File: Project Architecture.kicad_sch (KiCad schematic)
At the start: 0 parts

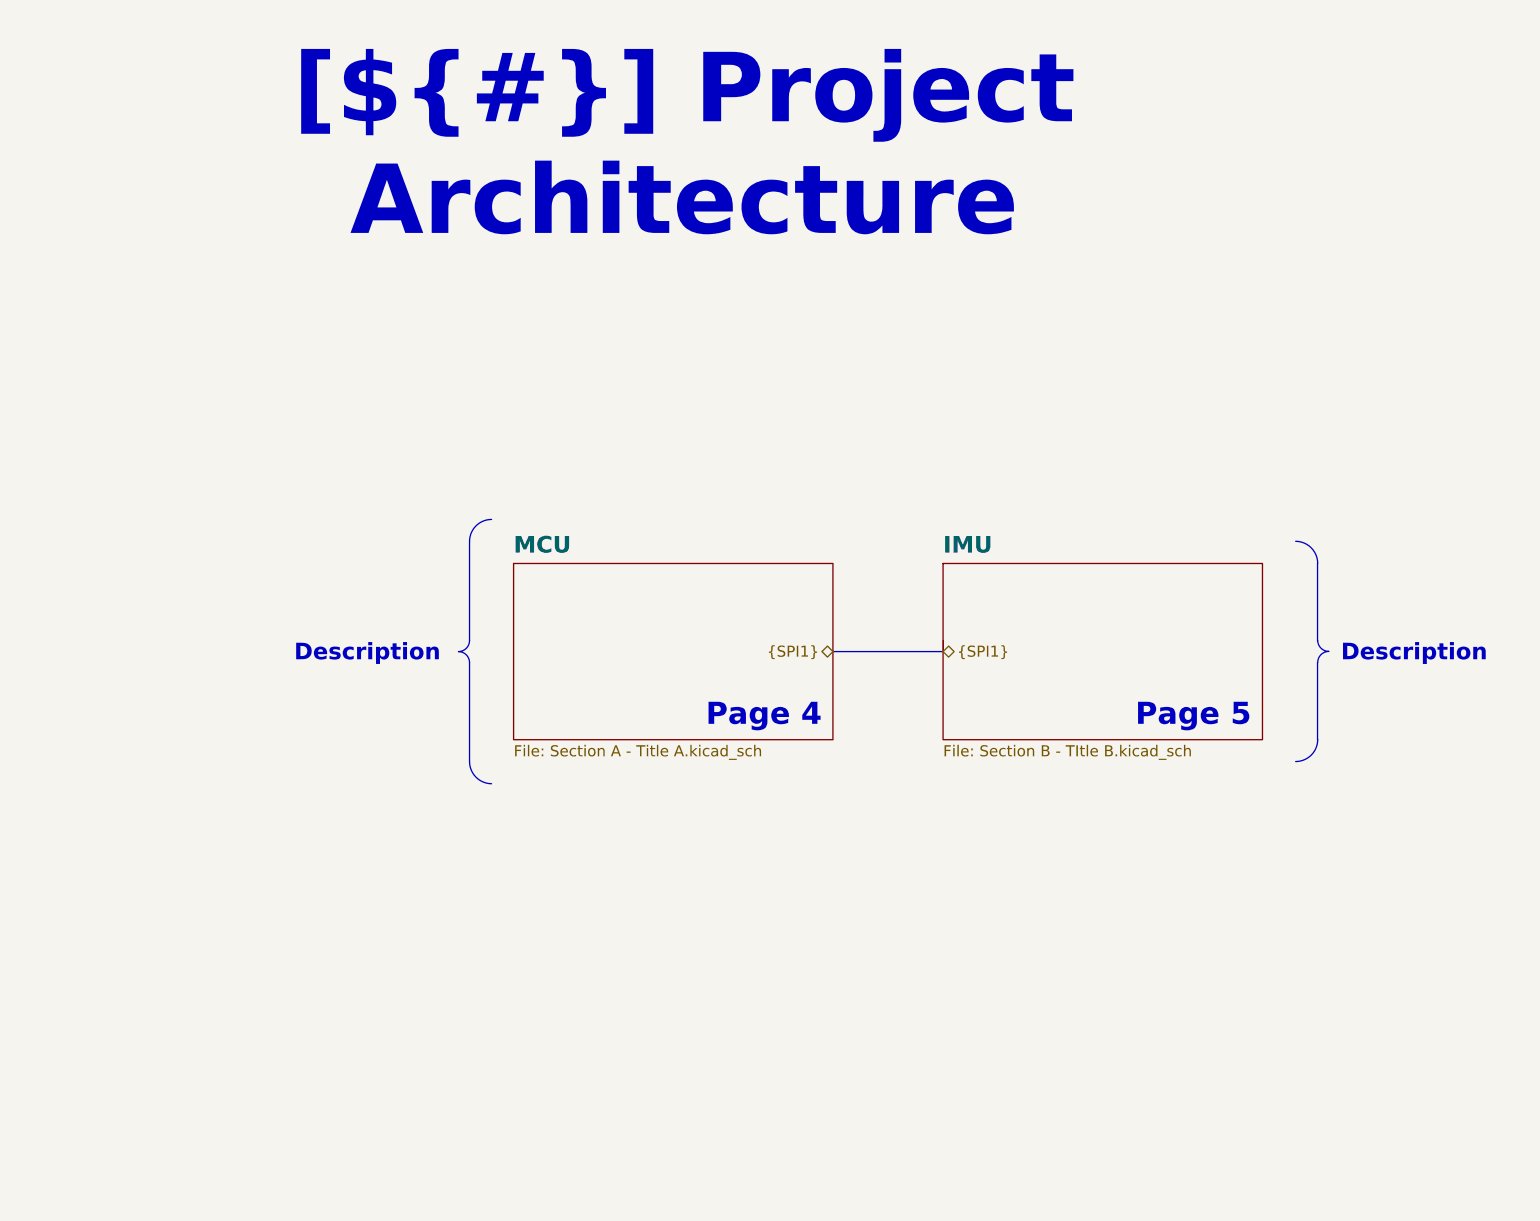
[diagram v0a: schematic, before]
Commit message: Schematic work & cleanup
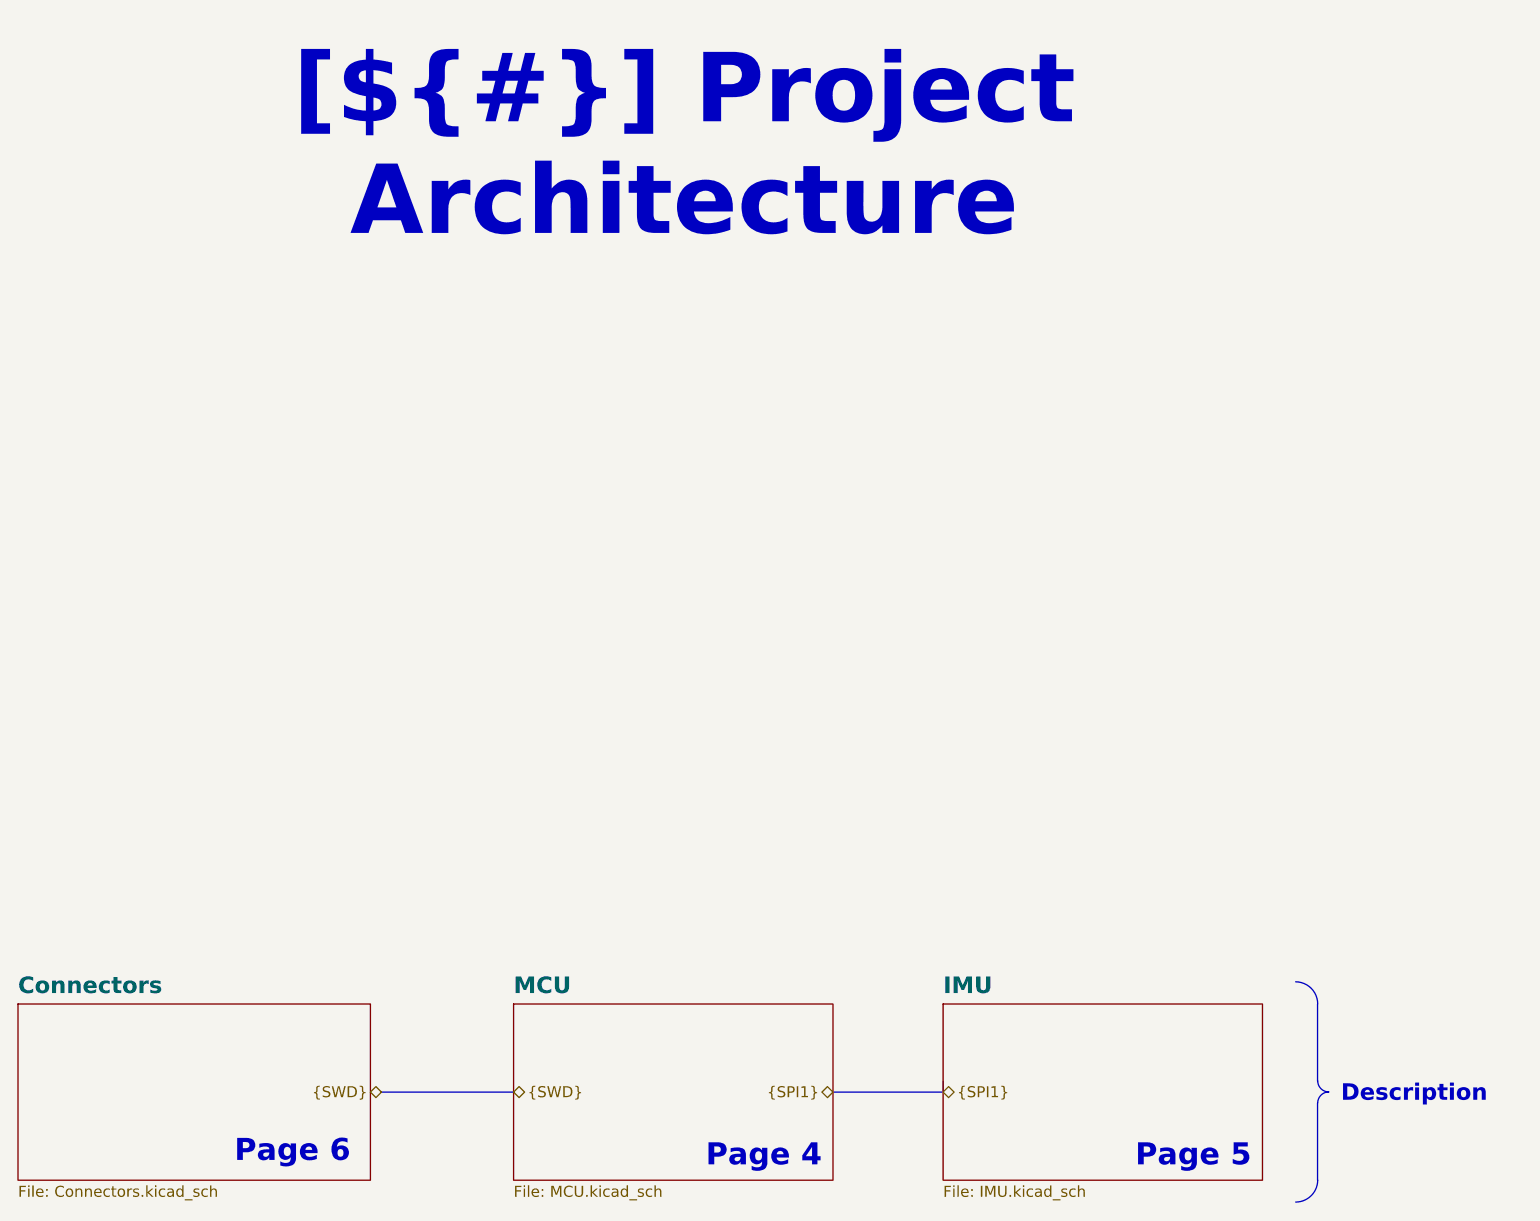
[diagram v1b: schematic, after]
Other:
- added sheet Connectors (Connectors.kicad_sch)
- sheet IMU: file Section B - TItle B.kicad_sch -> IMU.kicad_sch
- sheet MCU: file Section A - Title A.kicad_sch -> MCU.kicad_sch
- note added: "Page 6"
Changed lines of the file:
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@@
 	)
 	(arc
-		(start 185.42 85.09)
-		(mid 185.0451 85.9851)
-		(end 184.15 86.36)
+		(start 284.5 137.14)
+		(mid 283.6049 136.7651)
+		(end 283.23 135.87)
 		(stroke
 			(width 0)
@@
 	)
 	(arc
-		(start 284.5 86.34)
-		(mid 283.6049 85.9651)
-		(end 283.23 85.07)
+		(start 283.23 138.41)
+		(mid 283.6049 137.5149)
+		(end 284.5 137.14)
 		(stroke
 			(width 0)
@@
 	)
 	(arc
-		(start 283.23 87.61)
-		(mid 283.6049 86.7149)
-		(end 284.5 86.34)
+		(start 283.23 147.3)
+		(mid 282.4861 149.0961)
+		(end 280.69 149.84)
 		(stroke
 			(width 0)
@@
 	)
 	(arc
-		(start 283.23 96.5)
-		(mid 282.4861 98.2961)
-		(end 280.69 99.04)
-		(stroke
-			(width 0)
-			(type default)
-		)
-		(fill
-			(type none)
-		)
-	)
-	(arc
-		(start 184.15 86.36)
-		(mid 185.0451 86.7349)
-		(end 185.42 87.63)
-		(stroke
-			(width 0)
-			(type default)
-		)
-		(fill
-			(type none)
-		)
-	)
-	(arc
-		(start 187.96 101.6)
-		(mid 186.1698 100.8502)
-		(end 185.42 99.06)
-		(stroke
-			(width 0)
-			(type default)
-		)
-		(fill
-			(type none)
-		)
-	)
-	(arc
-		(start 280.69 73.64)
-		(mid 282.4802 74.3898)
-		(end 283.23 76.18)
-		(stroke
-			(width 0)
-			(type default)
-		)
-		(fill
-			(type none)
-		)
-	)
-	(arc
-		(start 185.42 73.66)
-		(mid 186.1639 71.8639)
-		(end 187.96 71.12)
-		(stroke
-			(width 0)
-			(type default)
-		)
-		(fill
-			(type none)
+		(start 280.69 124.44)
+		(mid 282.4802 125.1898)
+		(end 283.23 126.98)
+		(stroke
+			(width 0)
+			(type default)
+		)
+		(fill
+			(type none)
+		)
+	)
+	(text "Page 6"
+		(exclude_from_sim no)
+		(at 171.704 145.542 0)
+		(effects
+			(font
+				(size 2.54 2.54)
+				(bold yes)
+				(color 20 60 40 1)
+			)
+			(justify right bottom)
+			(href "#4")
 		)
 	)
 	(text "Page 5"
 		(exclude_from_sim no)
-		(at 275.59 95.25 0)
+		(at 275.59 146.05 0)
 		(effects
 			(font
@@
 	(text "Page 4"
 		(exclude_from_sim no)
-		(at 226.06 95.25 0)
+		(at 226.06 146.05 0)
 		(effects
 			(font
@@
 	(text_box "Description"
 		(exclude_from_sim no)
-		(at 166.37 83.82 0)
-		(size 17.145 5.08)
-		(margins 1.4287 1.4287 1.4287 1.4287)
-		(stroke
-			(width -0.0001)
-			(type default)
-		)
-		(fill
-			(type none)
-		)
-		(effects
-			(font
-				(size 1.905 1.905)
-				(thickness 0.381)
-				(bold yes)
-				(color 0 0 0 1)
-			)
-			(justify right top)
-		)
-	)
-	(text_box "Description"
-		(exclude_from_sim no)
-		(at 284.48 83.82 0)
+		(at 284.48 134.62 0)
 		(size 26.015 5.1)
 		(margins 1.4287 1.4287 1.4287 1.4287)
@@
 		)
 	)
+	(bus
+		(pts
+			(xy 175.26 137.16) (xy 190.5 137.16)
+		)
+		(stroke
+			(width 0)
+			(type default)
+		)
+	)
 	(polyline
 		(pts
-			(xy 240.03 85.09) (xy 240.03 86.36)
+			(xy 240.03 135.89) (xy 240.03 137.16)
 		)
 		(stroke
@@
 	(polyline
 		(pts
-			(xy 185.42 87.63) (xy 185.42 99.06)
+			(xy 283.21 138.43) (xy 283.21 147.32)
 		)
 		(stroke
@@
 	(polyline
 		(pts
-			(xy 283.21 87.63) (xy 283.21 96.52)
-		)
-		(stroke
-			(width 0)
-			(type default)
-		)
-	)
-	(polyline
-		(pts
-			(xy 185.42 85.09) (xy 185.42 73.66)
-		)
-		(stroke
-			(width 0)
-			(type default)
-		)
-	)
-	(polyline
-		(pts
-			(xy 283.21 76.2) (xy 283.21 85.09)
+			(xy 283.21 127) (xy 283.21 135.89)
 		)
 		(stroke
@@
 	(bus
 		(pts
-			(xy 227.33 86.36) (xy 240.03 86.36)
+			(xy 227.33 137.16) (xy 240.03 137.16)
 		)
 		(stroke
@@
 	(hierarchical_label "{SPI1}"
 		(shape bidirectional)
-		(at 240.03 86.36 0)
+		(at 240.03 137.16 0)
+		(effects
+			(font
+				(size 1.27 1.27)
+			)
+			(justify left)
+		)
+	)
+	(hierarchical_label "{SWD}"
+		(shape bidirectional)
+		(at 175.26 137.16 180)
+		(effects
+			(font
+				(size 1.27 1.27)
+			)
+			(justify right)
+		)
+	)
+	(hierarchical_label "{SWD}"
+		(shape bidirectional)
+		(at 190.5 137.16 0)
 		(effects
 			(font
@@
 	(hierarchical_label "{SPI1}"
 		(shape bidirectional)
-		(at 227.33 86.36 180)
+		(at 227.33 137.16 180)
 		(effects
 			(font
@@
 	)
 	(sheet
-		(at 240.03 76.2)
-		(size 36.83 20.32)
+		(at 133.35 127)
+		(size 40.64 20.32)
 		(exclude_from_sim no)
 		(in_bom yes)
@@
 		)
 		(fill
+			(color 162 242 255 1.0000)
+		)
+		(property "Sheetname" "Connectors"
+			(at 133.35 125.9709 0)
+			(effects
+				(font
+					(size 1.905 1.905)
+					(thickness 0.381)
+					(bold yes)
+				)
+				(justify left bottom)
+			)
+		)
+		(property "Sheetfile" "Connectors.kicad_sch"
+			(at 133.35 147.9046 0)
+			(effects
+				(font
+					(size 1.27 1.27)
+				)
+				(justify left top)
+			)
+		)
+		(instances
+			(project "seismic_sensor"
+				(path "/f9e05184-c88b-4a88-ae9c-ab2bdb32be7c/c5103ceb-5325-4a84-a025-9638a412984e"
+					(page "6")
+				)
+			)
+		)
+	)
+	(sheet
+		(at 240.03 127)
+		(size 36.83 20.32)
+		(exclude_from_sim no)
+		(in_bom yes)
+		(on_board yes)
+		(dnp no)
+		(fields_autoplaced yes)
+		(stroke
+			(width 0.1524)
+			(type solid)
+		)
+		(fill
 			(color 255 200 0 0.5020)
 		)
 		(property "Sheetname" "IMU"
-			(at 240.03 75.1709 0)
+			(at 240.03 125.9709 0)
 			(effects
 				(font
@@
 			)
 		)
-		(property "Sheetfile" "Section B - TItle B.kicad_sch"
-			(at 240.03 97.1046 0)
+		(property "Sheetfile" "IMU.kicad_sch"
+			(at 240.03 147.9046 0)
 			(effects
 				(font
@@
 	)
 	(sheet
-		(at 190.5 76.2)
+		(at 190.5 127)
 		(size 36.83 20.32)
 		(exclude_from_sim no)
@@
 		)
 		(property "Sheetname" "MCU"
-			(at 190.5 75.1709 0)
+			(at 190.5 125.9709 0)
 			(effects
 				(font
@@
 			)
 		)
-		(property "Sheetfile" "Section A - Title A.kicad_sch"
-			(at 190.5 97.1046 0)
-			(effects
-				(font
+		(property "Sheetfile" "MCU.kicad_sch"
+			(at 190.5 147.9046 0)
+			(effects
+				(font
